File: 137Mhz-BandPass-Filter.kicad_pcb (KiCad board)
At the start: 2 copper layers, 53 x 20 mm, 16 parts, among them J1 Conn_01x01, J2 Conn_01x01, J3 Conn_01x01, J4 Conn_01x01

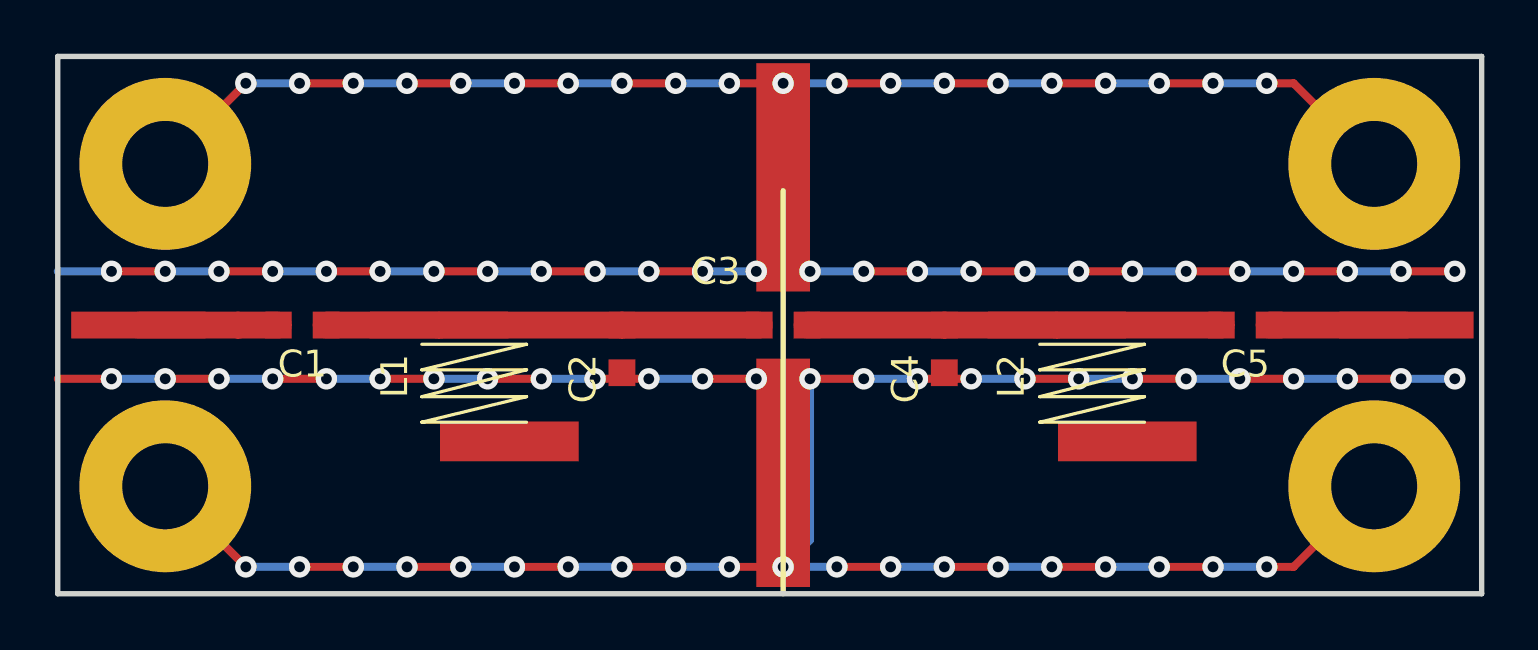
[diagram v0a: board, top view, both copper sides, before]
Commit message: Revision 2 done.
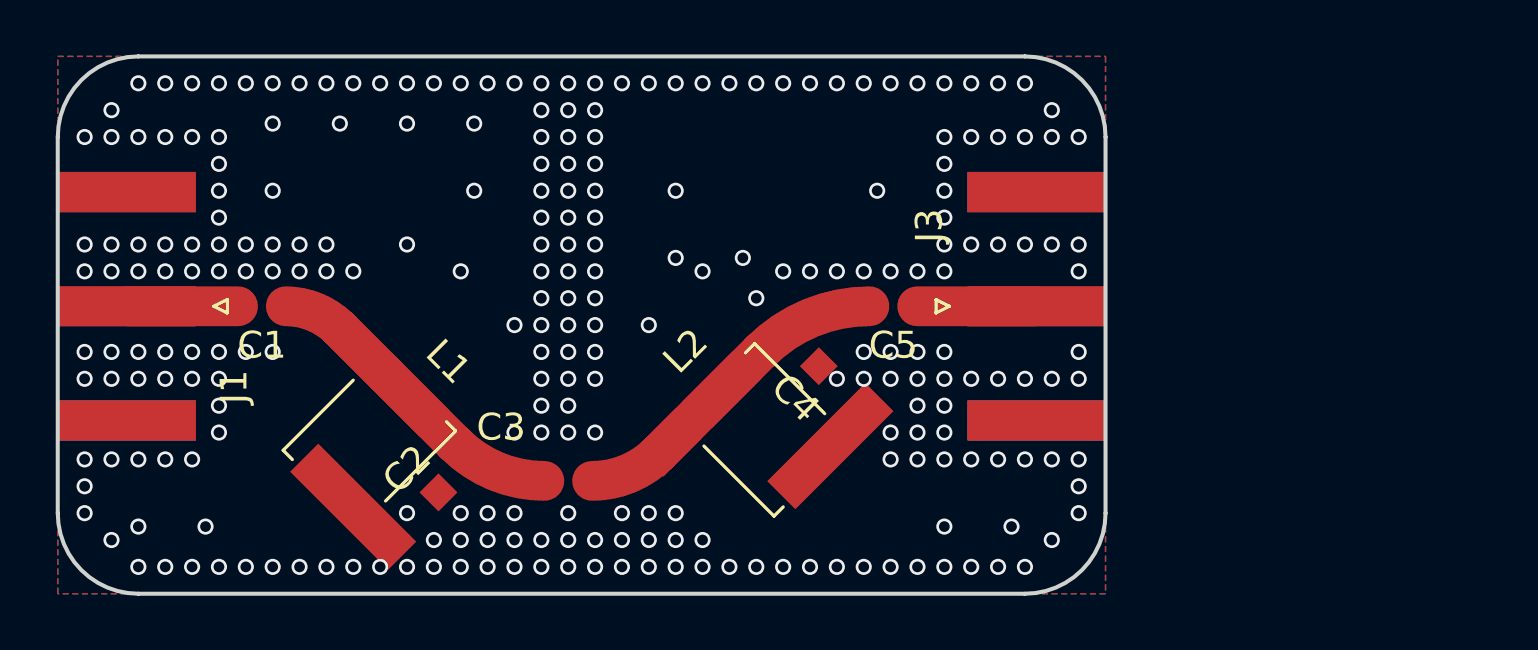
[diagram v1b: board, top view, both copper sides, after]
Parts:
- removed the G*** at (122.0, 120.0)
- removed J2, J4: Conn_01x01, Measurement_Points:Measurement_Point_Square-SMD-Pad_Big
- removed MK1, MK2, MK3, MK4: Mounting_Hole_PAD, MountingHole:MountingHole_3.2mm_M3_Pad
- added G***: LOGO, riske:NOAA_logo, F.Cu at (134.0, 115.0)
- added G***: LOGO, riske:logo_galaxy, B.Cu at (134.7, 114.5)
- C1, C5: value 4p7 -> 12p
- C2, C4: value 15p -> 27p
- C3: value 1p -> 4p7
- J1, J3: value Conn_01x01 -> Conn_Coaxial; footprint Connector_Wire:SolderWirePad_1x01_SMD_5x10mm -> Connector_Coaxial:SMA_Amphenol_132289_EdgeMount
- L1, L2: value 68n -> 33n; footprint kicad-footprints-master:Wurth-WE-CAIR-AirCoil-4,83x3,81 -> riske:L_Wurth_WE-CAIR-4248
- moved J3 13.8 mm to (143.4, 119.3), turned to 0 degrees
- moved C5 13.1 mm to (138.1, 119.3)
- moved L2 12.3 mm to (133.3, 123.9), turned to 45 degrees
- moved C3 9.88 mm to (126.0, 125.8)
- moved C2 7.79 mm to (121.8, 125.6), turned to 45 degrees
- moved C4 5.30 mm to (134.7, 120.9), turned to 135 degrees
- moved L1 4.45 mm to (118.6, 124.3), turned to -45 degrees
- moved C1 1.66 mm to (114.6, 119.3)
- moved J1 0.81 mm to (109.6, 119.3), turned to 180 degrees
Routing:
- net GND: track 206.4 -> 0.00 mm, vias 92 -> 256
- net Net-(C1-Pad1): track 16.1 -> 12.0 mm
- net Net-(C3-Pad1): track 15.4 -> 12.0 mm
- net Net-(J1-In): track 5.21 -> 4.11 mm
- net Net-(J3-In): track 5.11 -> 4.41 mm
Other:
- board size 53 x 20 mm -> 39 x 20 mm
- net class Default removed
- board text added: "137MHz BPF R2"
- board text removed: "137 MHz Band-pass filter"
